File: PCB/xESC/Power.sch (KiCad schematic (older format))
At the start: 23 parts, among them U2 TMC6100-LA, U3 LMV321, U4 MIC5504-1.8YM5

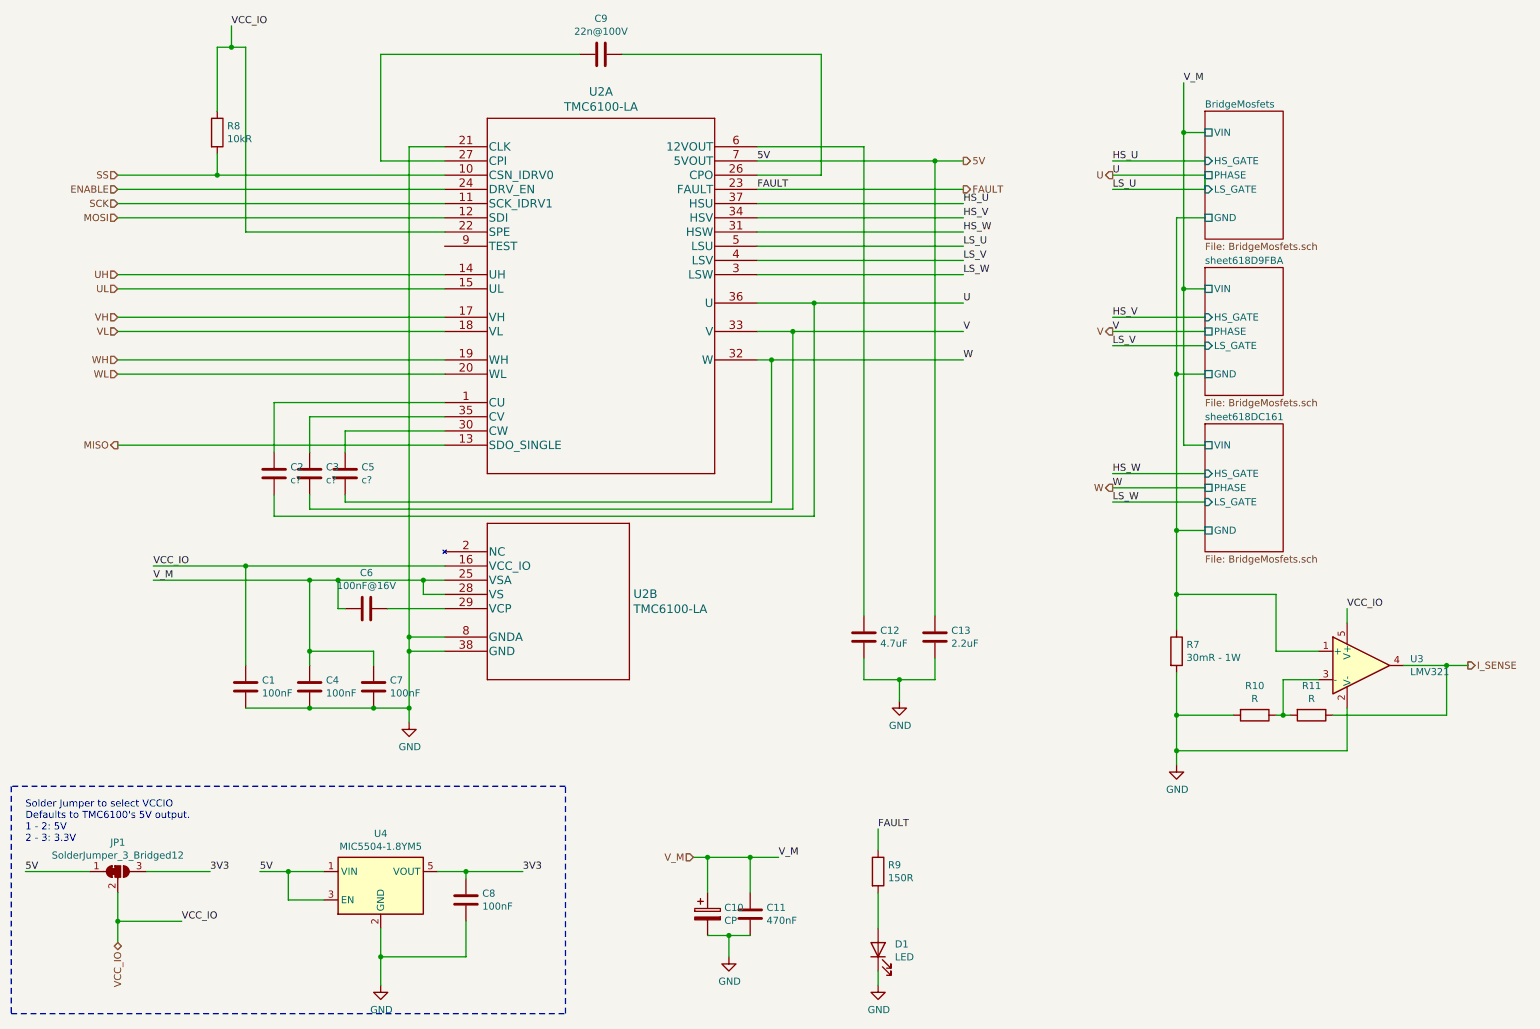
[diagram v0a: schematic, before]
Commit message: wip
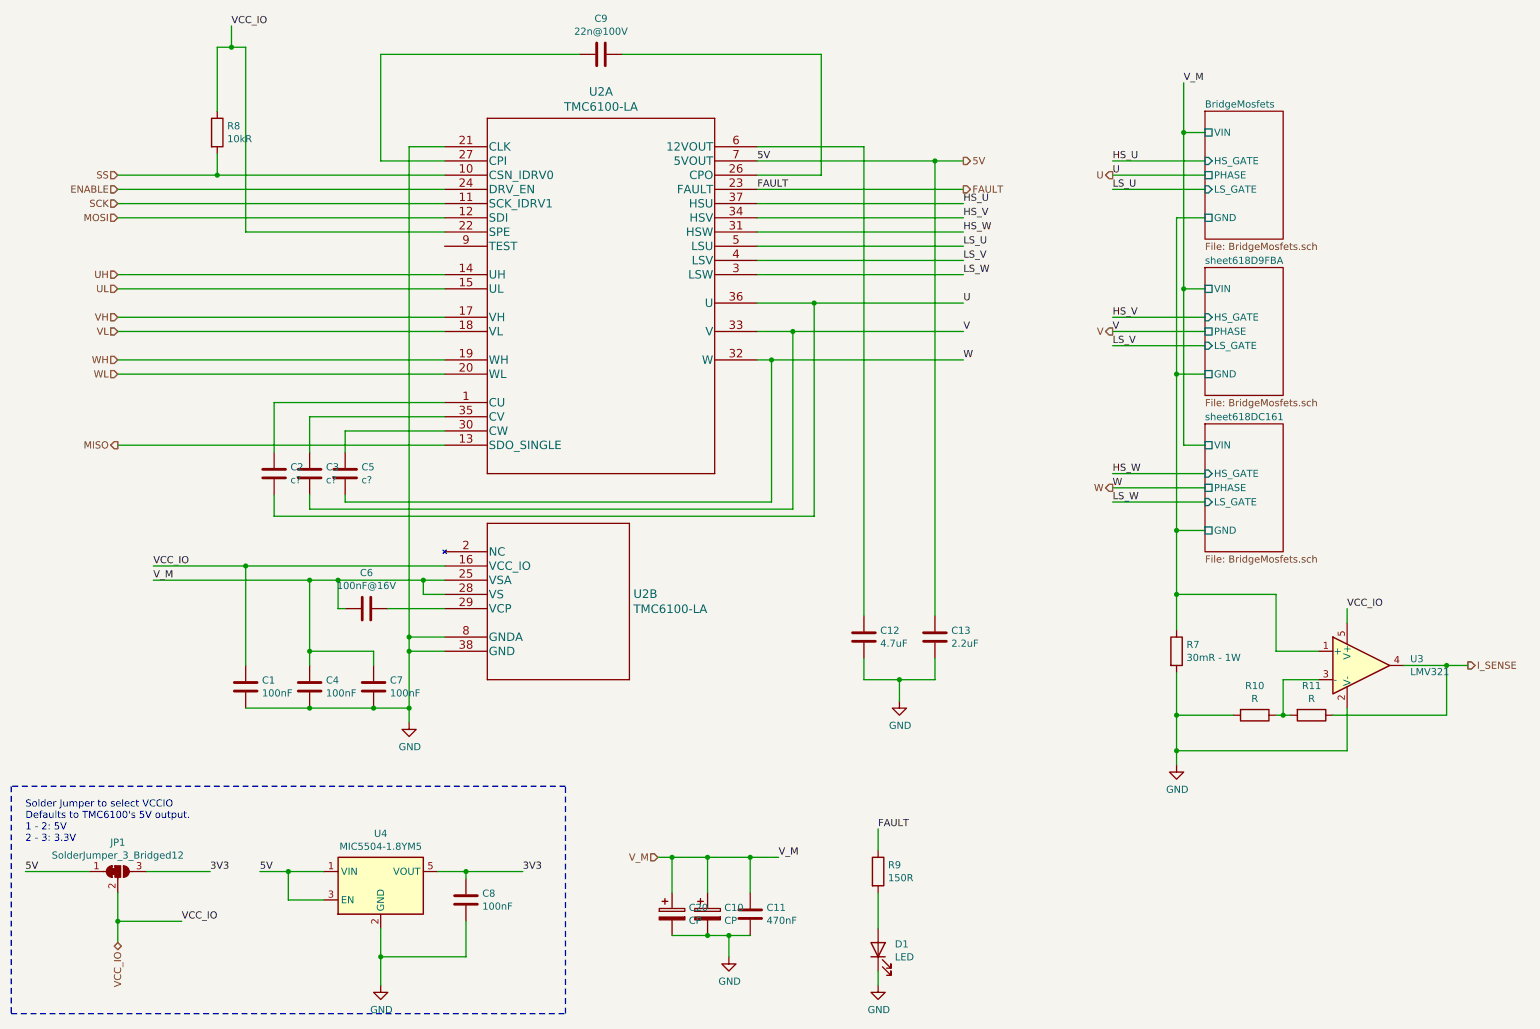
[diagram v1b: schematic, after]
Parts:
- added C20: CP, Capacitor_THT:CP_Radial_D8.0mm_P3.50mm, symbol Device:CP
- C1, C11, C12, C13, C2, C3, C4, C5, C6, C7, C8, C9: footprint (none) -> Capacitor_SMD:C_0805_2012Metric_Pad1.18x1.45mm_HandSolder
- C10: footprint (none) -> Capacitor_THT:CP_Radial_D8.0mm_P3.50mm
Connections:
- net GND: now also C20.2
- net U: no longer U2.5 (LSU)
- net V_M: now also C20.1
- new net LS_U: U2.5 (LSU)
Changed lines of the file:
@@
 	1    0    0    -1
 $EndComp
-Text HLabel 5350 6650 0    50   Input ~ 0
+Text HLabel 5100 6650 0    50   Input ~ 0
 V_M
 Wire Wire Line
@@
 F 0 "C4" H 2765 5496 50  0000 L CNN
 F 1 "100nF" H 2765 5405 50  0000 L CNN
-F 2 "" H 2688 5300 50  0001 C CNN
+F 2 "Capacitor_SMD:C_0805_2012Metric_Pad1.18x1.45mm_HandSolder" H 2688 5300 50  0001 C CNN
 F 3 "~" H 2650 5450 50  0001 C CNN
 	1    2650 5450
@@
 F 0 "C12" H 6665 5146 50  0000 L CNN
 F 1 "4.7uF" H 6665 5055 50  0000 L CNN
-F 2 "" H 6588 4950 50  0001 C CNN
+F 2 "Capacitor_SMD:C_0805_2012Metric_Pad1.18x1.45mm_HandSolder" H 6588 4950 50  0001 C CNN
 F 3 "~" H 6550 5100 50  0001 C CNN
 	1    6550 5100
@@
 F 0 "C1" H 2315 5496 50  0000 L CNN
 F 1 "100nF" H 2315 5405 50  0000 L CNN
-F 2 "" H 2238 5300 50  0001 C CNN
+F 2 "Capacitor_SMD:C_0805_2012Metric_Pad1.18x1.45mm_HandSolder" H 2238 5300 50  0001 C CNN
 F 3 "~" H 2200 5450 50  0001 C CNN
 	1    2200 5450
@@
 F 0 "C6" V 2798 4900 50  0000 C CNN
 F 1 "100nF@16V" V 2889 4900 50  0000 C CNN
-F 2 "" H 3088 4750 50  0001 C CNN
+F 2 "Capacitor_SMD:C_0805_2012Metric_Pad1.18x1.45mm_HandSolder" H 3088 4750 50  0001 C CNN
 F 3 "~" H 3050 4900 50  0001 C CNN
 	1    3050 4900
@@
 Wire Wire Line
 	2850 4700 2650 4700
-Wire Wire Line
-	5350 6650 5450 6650
 Text Label 5950 6650 0    50   ~ 0
 V_M
@@
 F 0 "C10" H 5568 7096 50  0000 L CNN
 F 1 "CP" H 5568 7005 50  0000 L CNN
-F 2 "" H 5488 6900 50  0001 C CNN
+F 2 "Capacitor_THT:CP_Radial_D8.0mm_P3.50mm" H 5488 6900 50  0001 C CNN
 F 3 "~" H 5450 7050 50  0001 C CNN
 	1    5450 7050
@@
 F 0 "C11" H 5865 7096 50  0000 L CNN
 F 1 "470nF" H 5865 7005 50  0000 L CNN
-F 2 "" H 5788 6900 50  0001 C CNN
+F 2 "Capacitor_SMD:C_0805_2012Metric_Pad1.18x1.45mm_HandSolder" H 5788 6900 50  0001 C CNN
 F 3 "~" H 5750 7050 50  0001 C CNN
 	1    5750 7050
@@
 F 0 "C7" H 3215 5496 50  0000 L CNN
 F 1 "100nF" H 3215 5405 50  0000 L CNN
-F 2 "" H 3138 5300 50  0001 C CNN
+F 2 "Capacitor_SMD:C_0805_2012Metric_Pad1.18x1.45mm_HandSolder" H 3138 5300 50  0001 C CNN
 F 3 "~" H 3100 5450 50  0001 C CNN
 	1    3100 5450
@@
 F 0 "C5" H 3015 3996 50  0000 L CNN
 F 1 "c?" H 3015 3905 50  0000 L CNN
-F 2 "" H 2938 3800 50  0001 C CNN
+F 2 "Capacitor_SMD:C_0805_2012Metric_Pad1.18x1.45mm_HandSolder" H 2938 3800 50  0001 C CNN
 F 3 "~" H 2900 3950 50  0001 C CNN
 	1    2900 3950
@@
 F 0 "C3" H 2765 3996 50  0000 L CNN
 F 1 "c?" H 2765 3905 50  0000 L CNN
-F 2 "" H 2688 3800 50  0001 C CNN
+F 2 "Capacitor_SMD:C_0805_2012Metric_Pad1.18x1.45mm_HandSolder" H 2688 3800 50  0001 C CNN
 F 3 "~" H 2650 3950 50  0001 C CNN
 	1    2650 3950
@@
 F 0 "C2" H 2515 3996 50  0000 L CNN
 F 1 "c?" H 2515 3905 50  0000 L CNN
-F 2 "" H 2438 3800 50  0001 C CNN
+F 2 "Capacitor_SMD:C_0805_2012Metric_Pad1.18x1.45mm_HandSolder" H 2438 3800 50  0001 C CNN
 F 3 "~" H 2400 3950 50  0001 C CNN
 	1    2400 3950
@@
 F 0 "C9" V 4952 1000 50  0000 C CNN
 F 1 "22n@100V" V 4861 1000 50  0000 C CNN
-F 2 "" H 4738 850 50  0001 C CNN
+F 2 "Capacitor_SMD:C_0805_2012Metric_Pad1.18x1.45mm_HandSolder" H 4738 850 50  0001 C CNN
 F 3 "~" H 4700 1000 50  0001 C CNN
 	1    4700 1000
@@
 F 0 "C13" H 7165 5146 50  0000 L CNN
 F 1 "2.2uF" H 7165 5055 50  0000 L CNN
-F 2 "" H 7088 4950 50  0001 C CNN
+F 2 "Capacitor_SMD:C_0805_2012Metric_Pad1.18x1.45mm_HandSolder" H 7088 4950 50  0001 C CNN
 F 3 "~" H 7050 5100 50  0001 C CNN
 	1    7050 5100
@@
 F 0 "C8" H 3865 6996 50  0000 L CNN
 F 1 "100nF" H 3865 6905 50  0000 L CNN
-F 2 "" H 3788 6800 50  0001 C CNN
+F 2 "Capacitor_SMD:C_0805_2012Metric_Pad1.18x1.45mm_HandSolder" H 3788 6800 50  0001 C CNN
 F 3 "~" H 3750 6950 50  0001 C CNN
 	1    3750 6950
@@
 	8950 1750 8300 1750
 Wire Wire Line
-	8950 1850 8950 1950
-Wire Wire Line
 	8950 1850 8300 1850
 Wire Wire Line
@@
 Text HLabel 8300 4050 0    50   Output ~ 0
 W
+$Comp
+L Device:CP C20
+U 1 1 61A2D5B8
+P 5200 7050
+F 0 "C20" H 5318 7096 50  0000 L CNN
+F 1 "CP" H 5318 7005 50  0000 L CNN
+F 2 "Capacitor_THT:CP_Radial_D8.0mm_P3.50mm" H 5238 6900 50  0001 C CNN
+F 3 "~" H 5200 7050 50  0001 C CNN
+	1    5200 7050
+	1    0    0    -1
+$EndComp
+Wire Wire Line
+	5100 6650 5200 6650
+Wire Wire Line
+	5200 6900 5200 6650
+Connection ~ 5200 6650
+Wire Wire Line
+	5200 6650 5450 6650
+Wire Wire Line
+	5200 7200 5450 7200
+Connection ~ 5450 7200
 $EndSCHEMATC

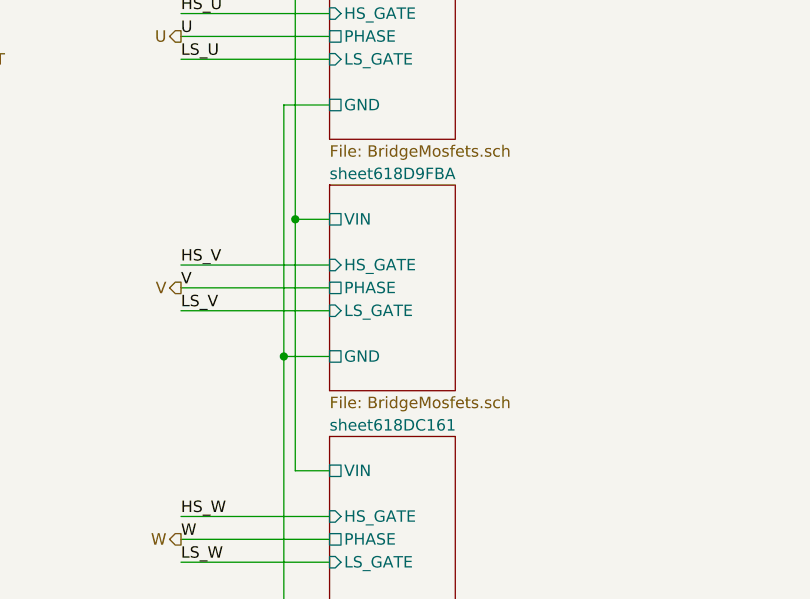
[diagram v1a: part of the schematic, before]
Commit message: wip
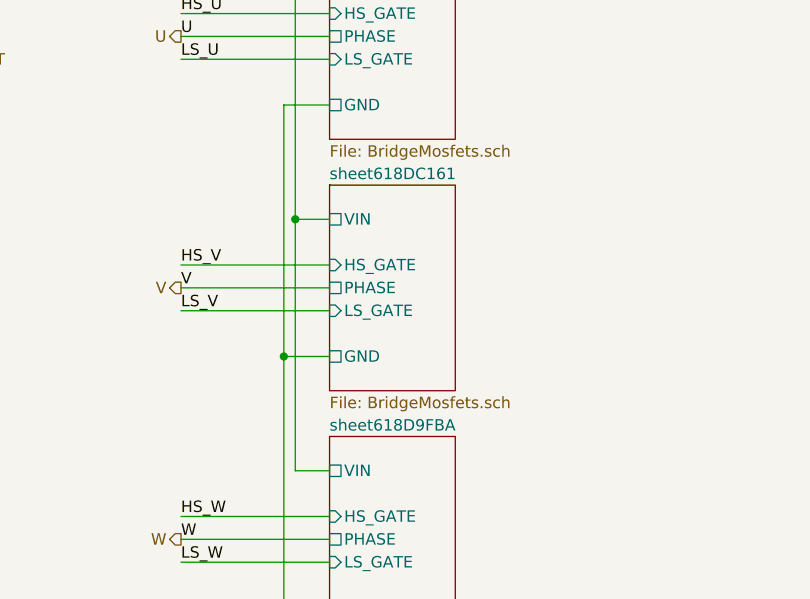
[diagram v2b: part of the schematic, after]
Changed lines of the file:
@@
 	4450 6150 550  6150
 $Sheet
-S 8950 2500 550  900
+S 8950 3600 550  900
 U 618D9FC1
 F0 "sheet618D9FBA" 50
+F1 "BridgeMosfets.sch" 50
+F2 "VIN" U L 8950 3750 50
+F3 "GND" U L 8950 4350 50
+F4 "PHASE" U L 8950 4050 50
+F5 "HS_GATE" I L 8950 3950 50
+F6 "LS_GATE" I L 8950 4150 50
+$EndSheet
+$Sheet
+S 8950 2500 550  900
+U 618DC168
+F0 "sheet618DC161" 50
 F1 "BridgeMosfets.sch" 50
 F2 "VIN" U L 8950 2650 50
@@
 F6 "LS_GATE" I L 8950 3050 50
 $EndSheet
-$Sheet
-S 8950 3600 550  900
-U 618DC168
-F0 "sheet618DC161" 50
-F1 "BridgeMosfets.sch" 50
-F2 "VIN" U L 8950 3750 50
-F3 "GND" U L 8950 4350 50
-F4 "PHASE" U L 8950 4050 50
-F5 "HS_GATE" I L 8950 3950 50
-F6 "LS_GATE" I L 8950 4150 50
-$EndSheet
 Wire Wire Line
